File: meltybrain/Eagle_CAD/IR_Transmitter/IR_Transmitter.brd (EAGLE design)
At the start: 30.9 x 28.5 mm, 14 parts, among them J1 AVR_SPI_PROG_3X2NS, Q1 BSS806N, Q2 FDN352AP, U1 LMH6612MAX/NOPB, U2 AP2210K-5.0TRG1, U3 ATTINY84

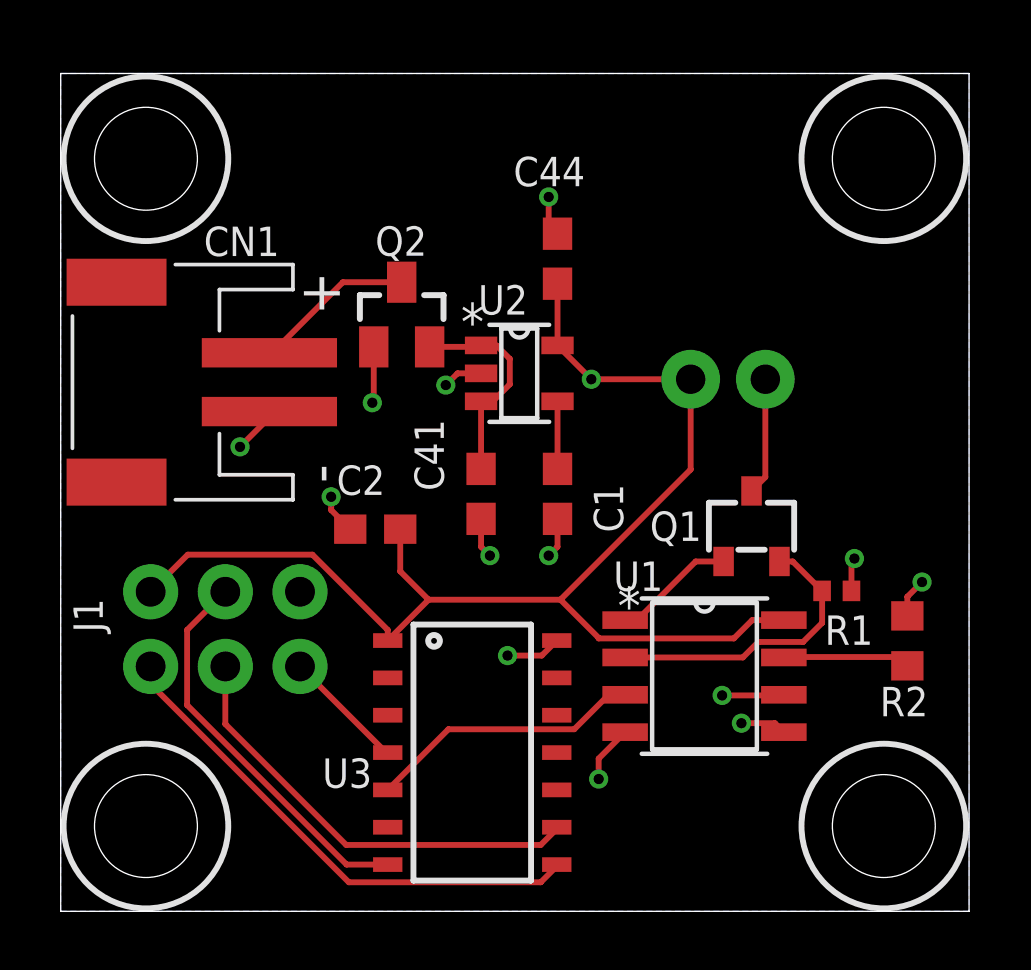
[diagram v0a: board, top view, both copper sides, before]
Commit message: second round of gerbers
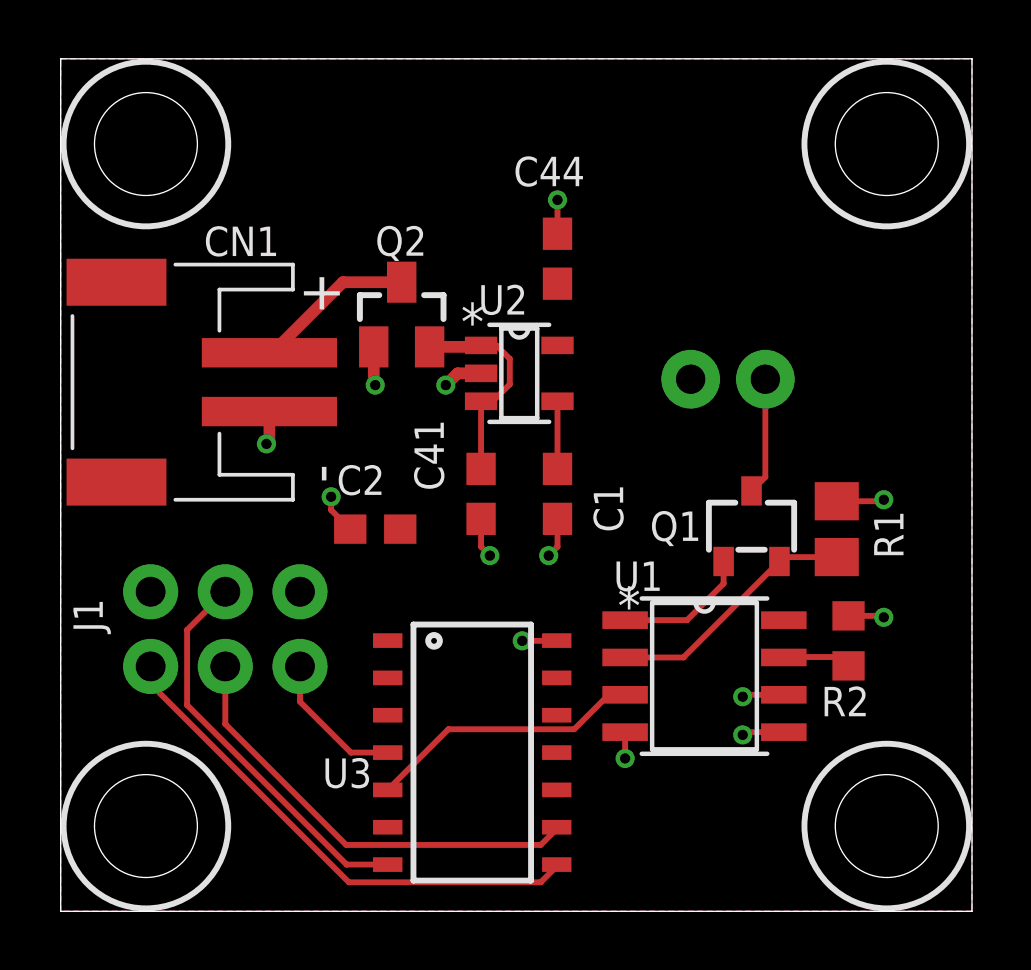
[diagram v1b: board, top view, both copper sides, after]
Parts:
- R1: device rcl:R0402 -> rcl:R0805
- moved R1 2.10 mm to (26.4, 13.0), turned to 270 degrees
- moved R2 2.00 mm to (26.8, 9.20)
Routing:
- net +5V: track 44.1 -> 0.00 mm, vias 1 -> 0
- net GND: track 20.5 -> 16.9 mm
- net N$3: track 4.48 -> 2.48 mm
- net N$1: track 10.1 -> 8.61 mm
- net RST: track 4.20 -> 4.90 mm
- added copper zone on layer 1, net +5V
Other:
- board size 30.9 x 28.5 mm -> 31 x 29 mm
